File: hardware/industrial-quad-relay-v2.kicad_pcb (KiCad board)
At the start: 2 copper layers, 40 x 40 mm, 36 parts, among them P1 CON-SENSOR, P2 Digital Output, P3 Debug, P4 Boot, U1 XMC1100, U2 CPC1002N, U3 CPC1002N, U4 CPC1002N, U5 CPC1002N, U6 DRILL, U7 DRILL, U8 DRILL, U9 DRILL

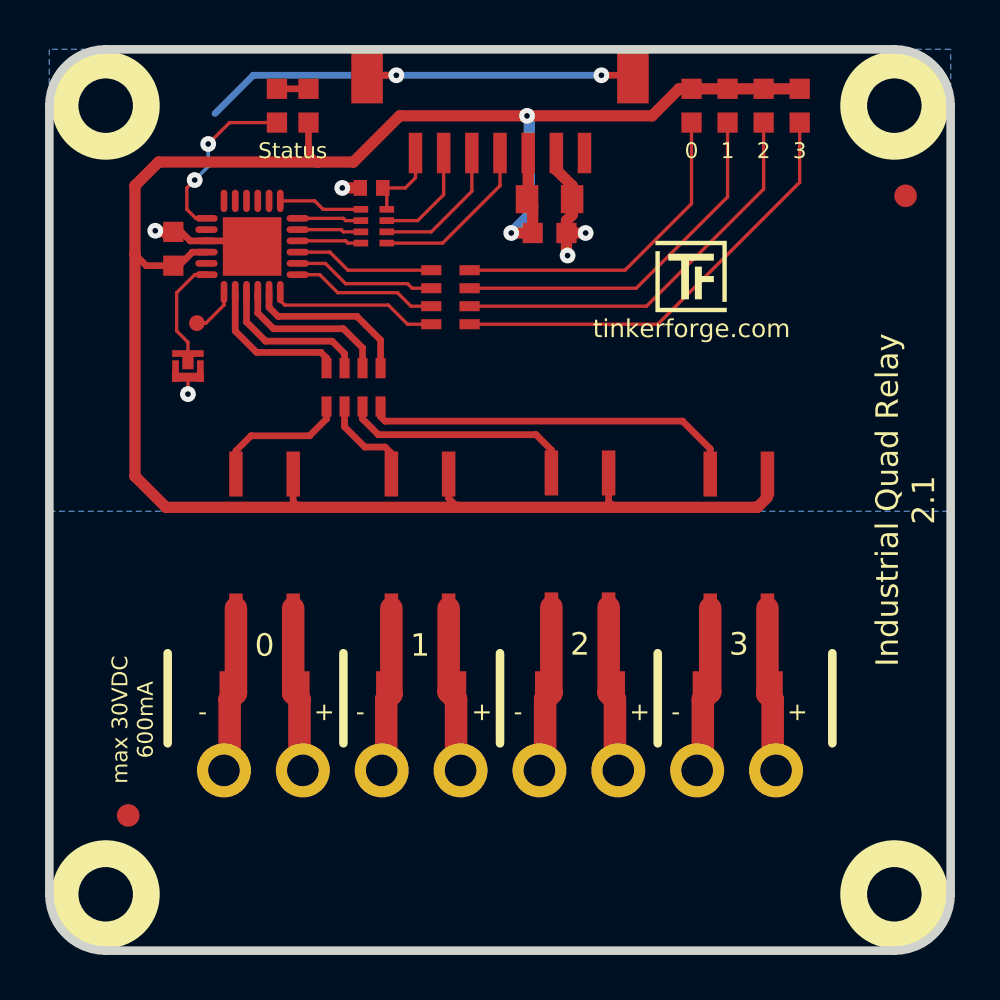
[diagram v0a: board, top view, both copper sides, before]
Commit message: move to new kicad version
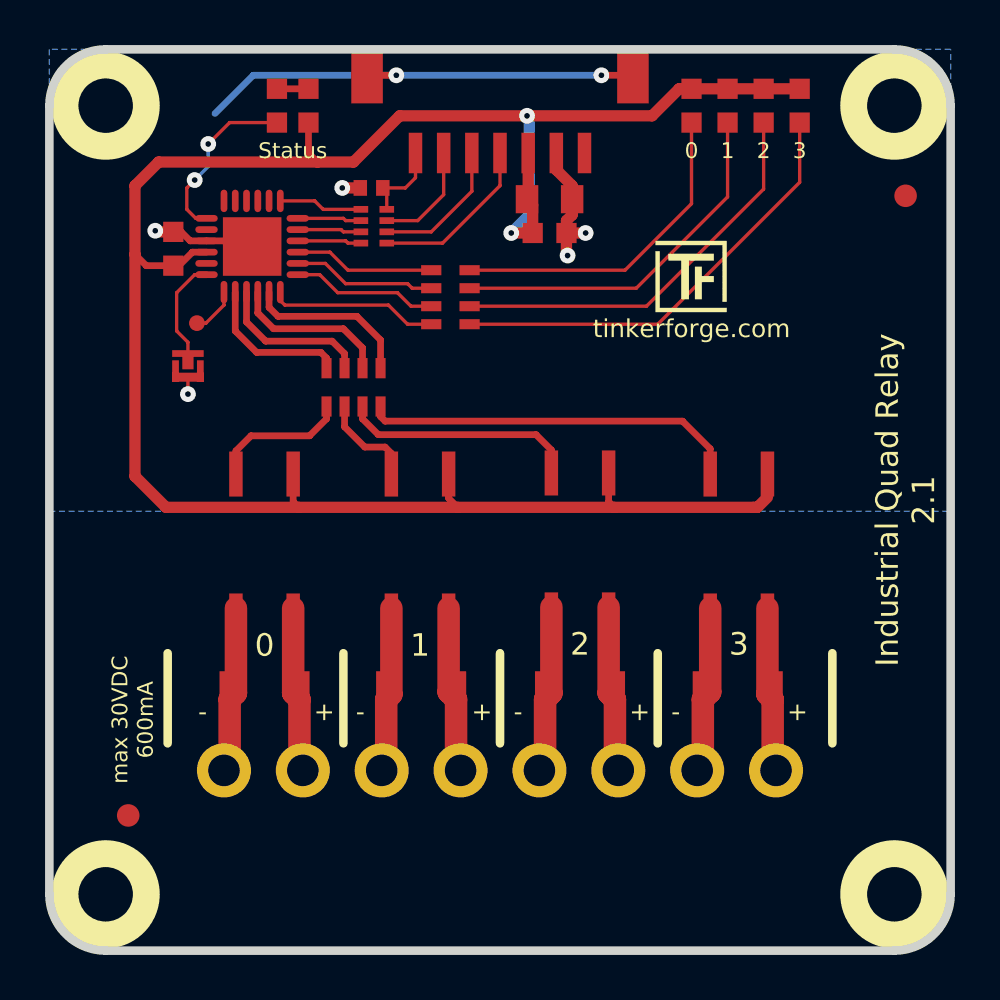
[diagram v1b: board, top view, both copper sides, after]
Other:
- net class Default removed
